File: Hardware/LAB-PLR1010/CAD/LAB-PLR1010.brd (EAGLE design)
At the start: 15.2 x 26.7 mm, 8 parts, among them IC1 LT1963AEQ, U1 AD5270BRMZ-50

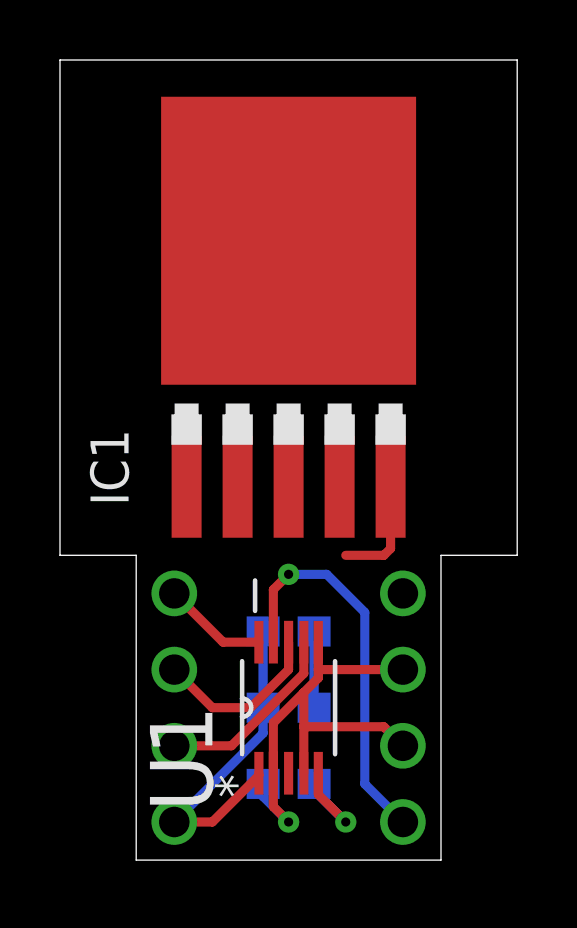
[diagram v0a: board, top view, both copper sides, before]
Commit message: 1) Updates to the LAB-PLR1010
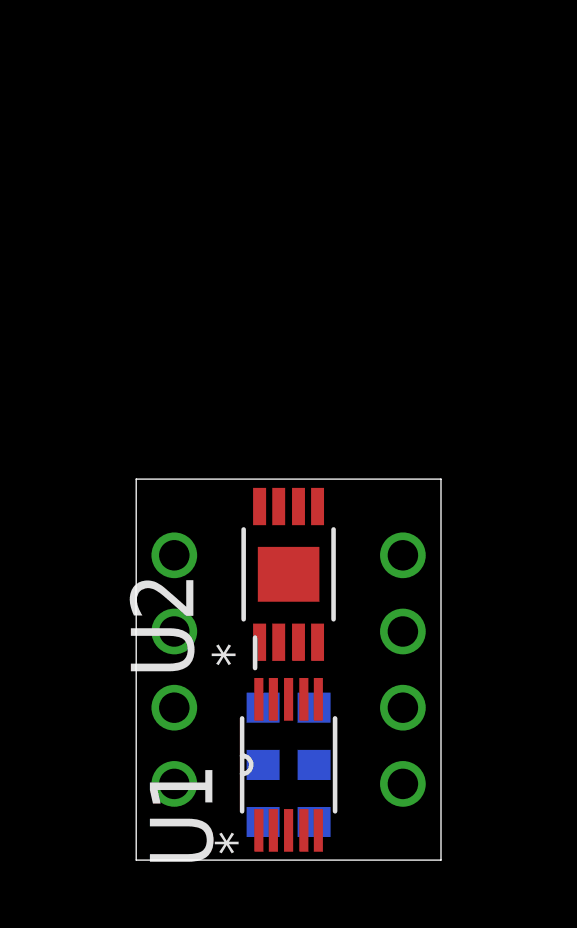
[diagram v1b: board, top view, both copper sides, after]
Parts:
- removed IC1: LT1963AEQ, linear-technology:Q5-DD
- removed R1: 1R0, rcl:R2512
- added U2: LT3080EMS8EPBF, LAB-PLR1010:SOP65P490X110-9N
- moved C3 2.54 mm to (5.08, 5.08)
- moved C2 1.91 mm to (5.08, 3.17)
- moved U1 1.91 mm to (5.08, 3.17)
- moved C1 1.27 mm to (5.08, 1.27)
- moved SV1 1.27 mm to (8.89, 6.35)
- moved SV2 1.27 mm to (1.27, 6.35)
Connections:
- removed net N$9: IC1.4, R1.2
- new net VOUT: SV1.3, U2.1, U2.2, U2.3, U2.9
- net N$8: now also U2.4; no longer IC1.5
- net PE: no longer IC1.3, IC1.6, R1.1, SV1.3
- net VDDIO: now also U2.5
- net VDDLDO: now also U2.7, U2.8; no longer IC1.1, IC1.2
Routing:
- net PE: track 20.1 -> 0.00 mm, vias 1 -> 0
- net MCLK: track 13.0 -> 0.00 mm, vias 1 -> 0
- net VDDIO: track 11.1 -> 0.00 mm
- net MISO: track 6.36 -> 0.00 mm
- net MOSI: track 5.78 -> 0.00 mm
- net N$1: track 3.71 -> 0.00 mm, vias 1 -> 0
- net N$8: track 3.65 -> 0.00 mm
- net #CS: track 3.49 -> 0.00 mm
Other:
- board size 15.2 x 26.7 mm -> 10.2 x 12.7 mm

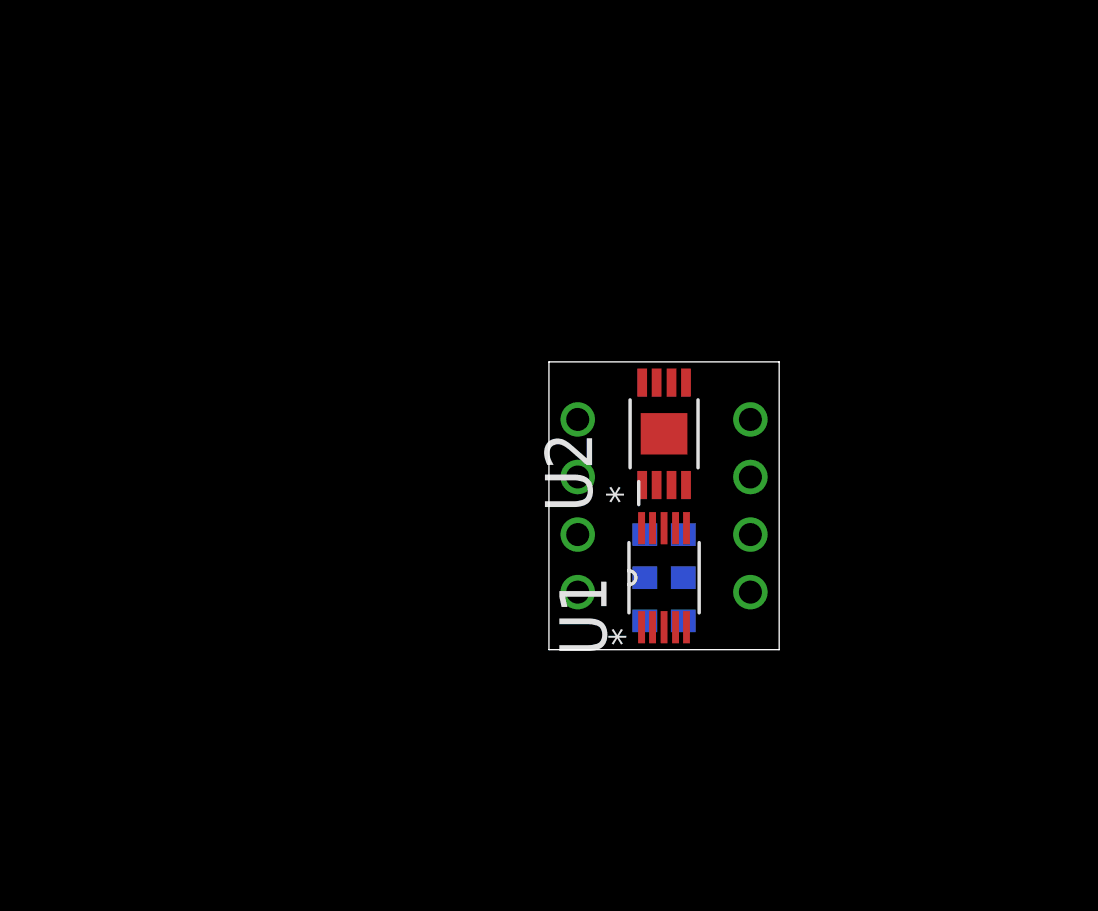
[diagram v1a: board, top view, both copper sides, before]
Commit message: 1) Updates to the PLR1010 + datasheet and bills of materials
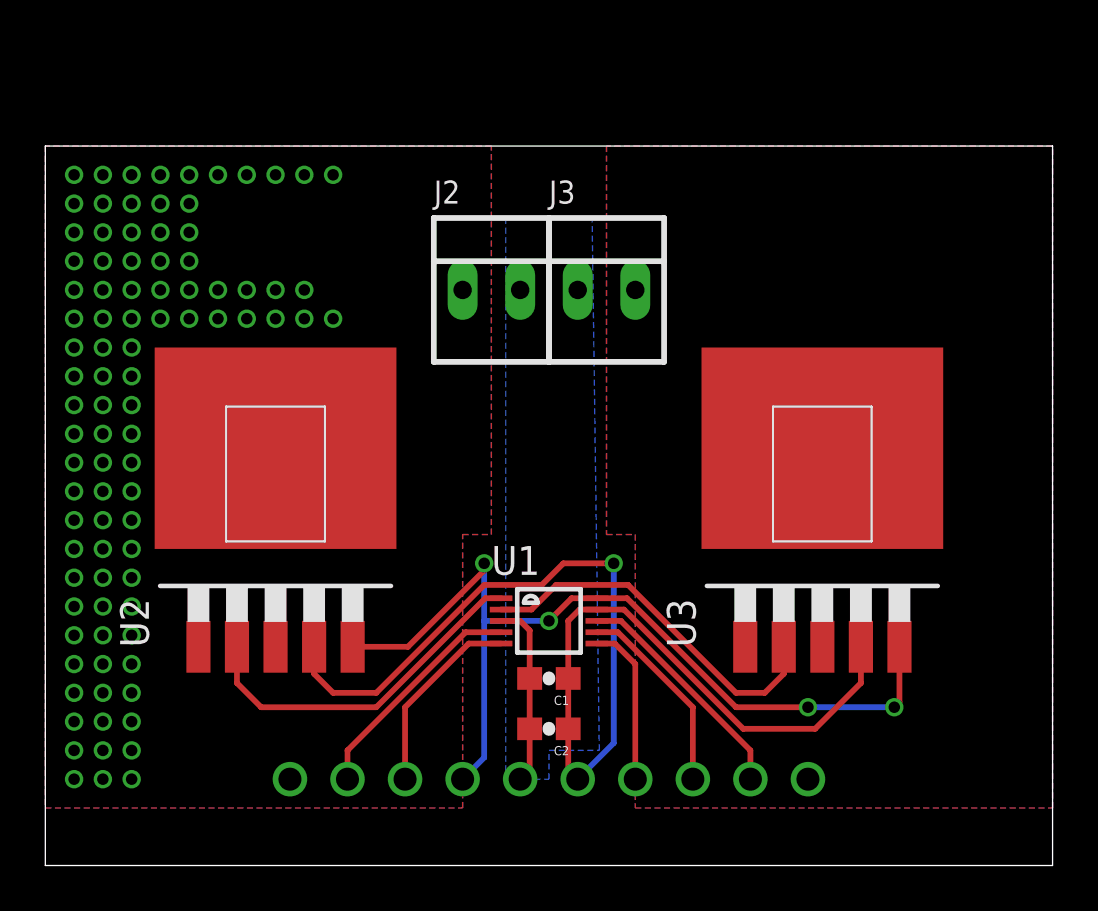
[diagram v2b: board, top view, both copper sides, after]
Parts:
- removed C3: 10uF, SparkFun-Capacitors:0603-CAP
- removed SV1, SV2: (no value), LAB304:MA04-1
- added J1: (no value), con-lstb:MA10-1W
- added J2, J3: 22-23-2021, My Library-adm:22-23-2021
- added U3: LT3080, LAB-PLR1010:DDPAK5(Q)
- C1: value 1uF -> 10uF
- U1: value AD5270BRMZ-50 -> DAC8562; device Analog Devices_By_element14_Batch_1:SOP50P490X110-10N -> LAB-PLR1010:MSOP10
- U2: value LT3080EMS8EPBF -> LT3080; device LAB-PLR1010:SOP65P490X110-9N -> LAB-PLR1010:DDPAK5(Q)
- moved U2 17.2 mm to (-12.1, 8.89), turned to 0 degrees
- moved C2 8.38 mm to (0.00, -3.49), flipped to the top
- moved C1 5.68 mm to (0.00, -1.27), flipped to the top, turned to 180 degrees
- moved U1 5.43 mm to (0.00, 1.27), turned to 270 degrees
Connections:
- removed net #CS: SV2.4, U1.10
- removed net MISO: SV2.2, U1.7
- removed net N$1: C1.1, U1.5
- removed net N$8: U1.3, U2.4
- removed net PE: C1.2, C2.2, C3.2, SV1.2, U1.2, U1.4, U1.6
- removed net VOUT: SV1.3, U2.1, U2.2, U2.3, U2.9
- new net !CLR: J1.3, U1.5
- new net !CS: J1.7, U1.6
- new net !LDAC: J1.2, U1.4
- new net GND: C1.2, C2.2, J1.5, J2.2, J3.1, U1.3
- new net N$2: U1.1, U2.2
- new net N$3: U1.2, U3.2
- new net VA: J1.1, J2.1, U2.3, U2.TAB
- new net VB: J1.10, J3.2, U3.3, U3.TAB
- net MCLK: now also J1.8, U1.7; no longer SV1.4, U1.9
- net MOSI: now also J1.9; no longer SV2.3
- net VDDIO: now also C1.1, J1.6, U1.9, U2.4, U3.4; no longer C3.1, SV2.1, U1.1, U2.5
- net VDDLDO: now also J1.4, U1.10, U2.5, U3.5; no longer SV1.1, U2.7, U2.8
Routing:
- net VDDIO: track 0.00 -> 52.2 mm, vias 0 -> 1
- net VDDLDO: track 0.00 -> 40.7 mm, vias 0 -> 4
- net N$3: track 0.00 -> 16.4 mm
- net N$2: track 0.00 -> 15.7 mm
- net MOSI: track 0.00 -> 10.4 mm
- net !LDAC: track 0.00 -> 10.2 mm
- net MCLK: track 0.00 -> 8.78 mm
- net !CLR: track 0.00 -> 8.58 mm
- net GND: track 0.00 -> 8.18 mm
- net !CS: track 0.00 -> 7.15 mm
- added copper zone on layer 16, net GND
- added copper zone on layer 1, net VA
- added copper zone on layer 16, net VA
- added copper zone on layer 1, net VB
- added copper zone on layer 16, net VB
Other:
- board size 10.2 x 12.7 mm -> 44.5 x 31.8 mm
